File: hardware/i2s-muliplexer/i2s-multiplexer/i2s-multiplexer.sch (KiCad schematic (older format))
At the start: 27 parts, among them J1 Conn_01x05, J2 Conn_01x05, J3 Conn_01x05, J4 Conn_01x05, J5 Conn_01x05, J6 Conn_01x07, J7 Conn_01x05, U1 74HC126, U2 74HC126, U3 74HC126, U4 74HC126, U5 74HC126, U6 74HC126, U7 74LS138

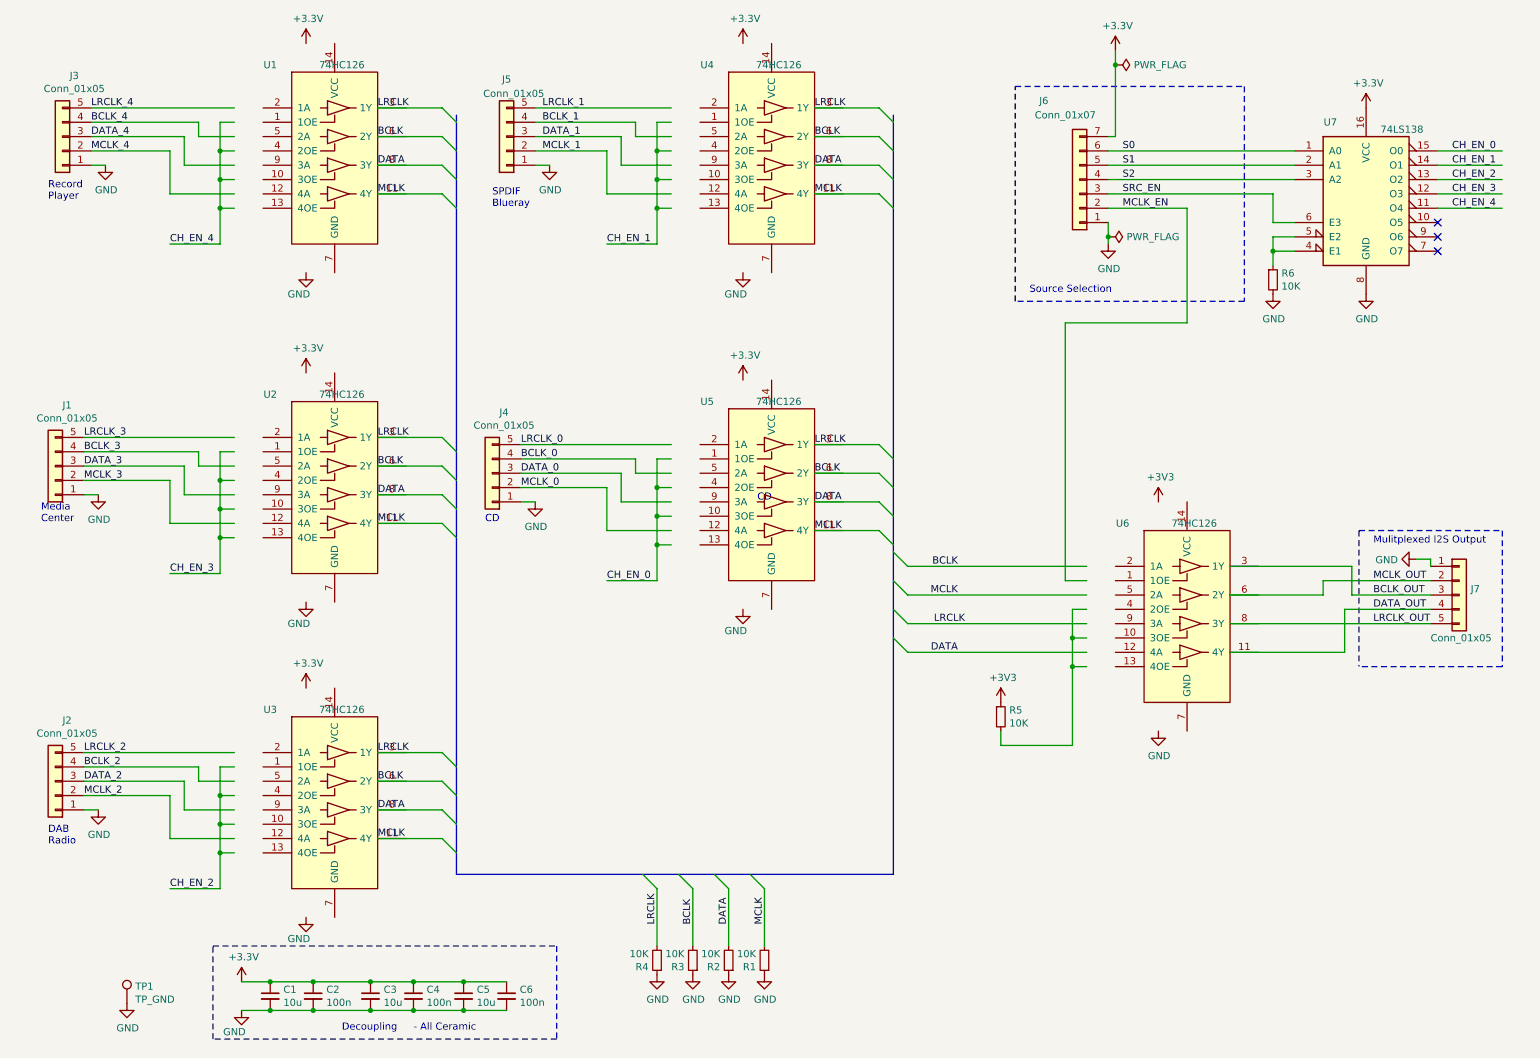
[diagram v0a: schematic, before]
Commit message: Initial placement
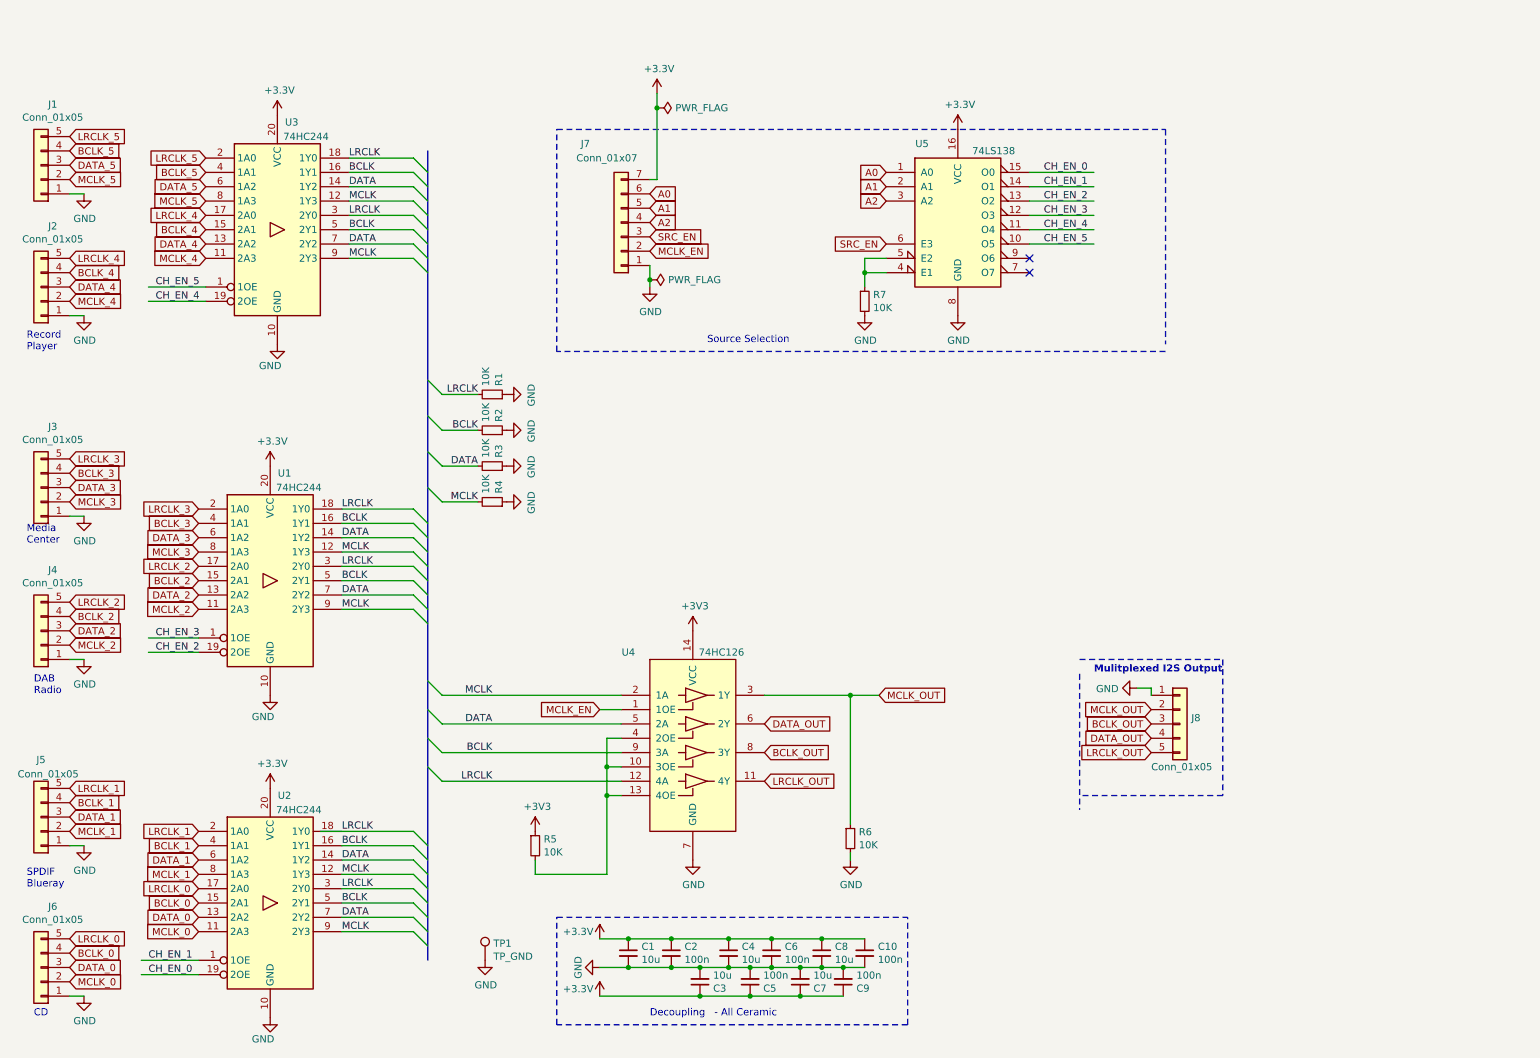
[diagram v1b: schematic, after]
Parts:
- removed U1, U2, U3, U4, U5: 74HC126, Package_SO:SOIC-14_3.9x8.7mm_P1.27mm, symbol i2s-multiplexer:74HC126
- added C3, C7: 10u, Capacitor_SMD:C_0805_2012Metric_Pad1.15x1.40mm_HandSolder, symbol Device:C_Small
- added C5, C9: 100n, Capacitor_SMD:C_0805_2012Metric_Pad1.15x1.40mm_HandSolder, symbol Device:C_Small
- added J1: Conn_01x05, Connector_PinHeader_2.54mm:PinHeader_1x05_P2.54mm_Vertical, symbol Connector_Generic:Conn_01x05
- added R6: 10K, Resistor_SMD:R_0805_2012Metric_Pad1.15x1.40mm_HandSolder, symbol Device:R_Small
- added U1, U2, U3: 74HC244, Package_SO:SOIC-20W_7.5x12.8mm_P1.27mm, symbol 74xx:74HC244
- C1, C2: footprint (none) -> Capacitor_SMD:C_0805_2012Metric_Pad1.15x1.40mm_HandSolder
- C10: renamed from C6; footprint (none) -> Capacitor_SMD:C_0805_2012Metric_Pad1.15x1.40mm_HandSolder
- C4: renamed from C3; footprint (none) -> Capacitor_SMD:C_0805_2012Metric_Pad1.15x1.40mm_HandSolder
- C6: renamed from C4; footprint (none) -> Capacitor_SMD:C_0805_2012Metric_Pad1.15x1.40mm_HandSolder
- C8: renamed from C5; footprint (none) -> Capacitor_SMD:C_0805_2012Metric_Pad1.15x1.40mm_HandSolder
- renumbered J3 to J2, J1 to J3, J2 to J4, J4 to J6, J6 to J7, J7 to J8, R4 to R1, R3 to R2, R2 to R3, R1 to R4, R6 to R7, U6 to U4, U7 to U5
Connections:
- net labels added: A0, A1, A2, BCLK_5, CH_EN_5, DATA_5, LRCLK_5, MCLK_5
- net labels removed: S0, S1, S2
- wire segments 185 -> 94
- no-connect marks 3 -> 2
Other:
- note removed: "CD"
- moved on the sheet: C1, C10, C2, C4, C6, C8, J2, J3, J4, J5, J6, J7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
